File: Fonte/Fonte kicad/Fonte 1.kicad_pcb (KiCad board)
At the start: 2 copper layers, 12 parts, among them J1 Screw_Terminal_01x03, Q1 BC547

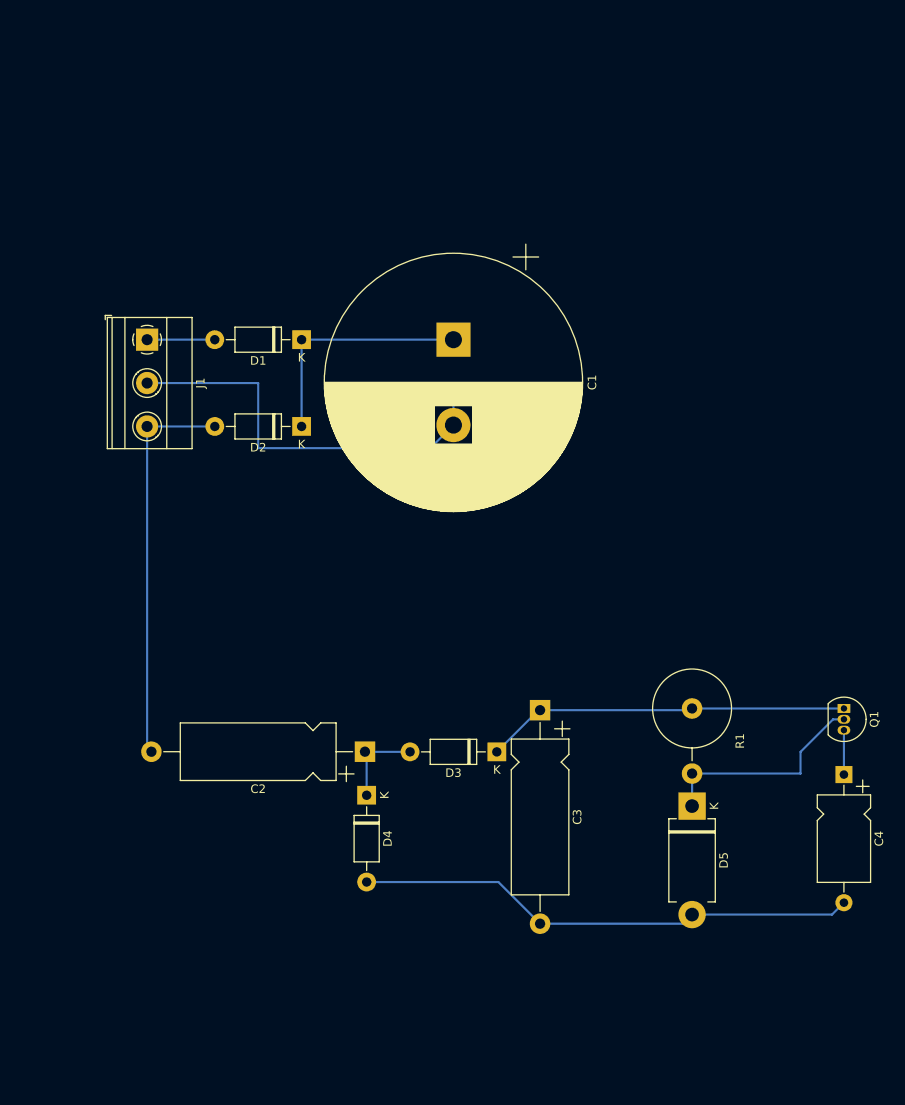
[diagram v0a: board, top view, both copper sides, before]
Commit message: Add files via upload
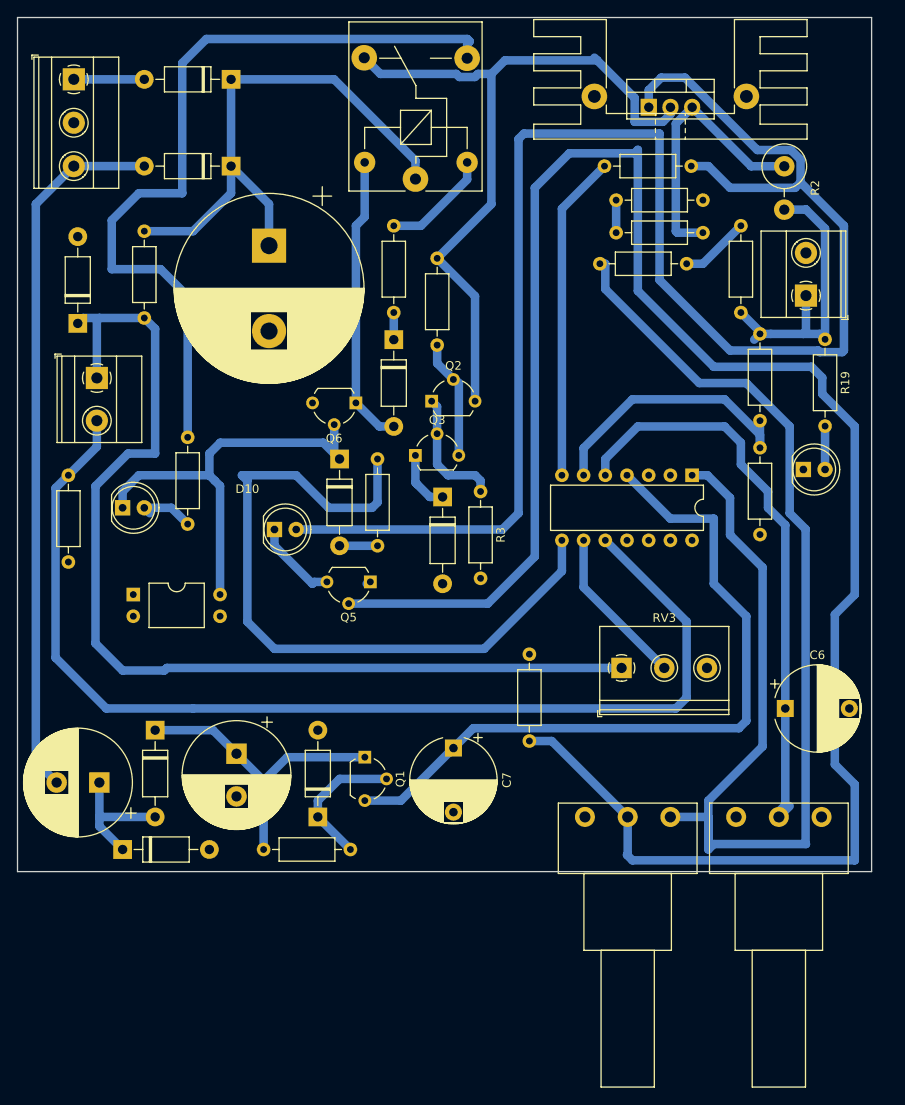
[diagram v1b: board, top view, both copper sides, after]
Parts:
- removed C4: 100n, Capacitor_THT:CP_Axial_L10.0mm_D6.0mm_P15.00mm_Horizontal
- added C6: 10u, Capacitor_THT:CP_Radial_D10.0mm_P7.50mm, F.Cu at (104.9, 88.9)
- added C7: 100n, Capacitor_THT:CP_Radial_D10.0mm_P7.50mm, F.Cu at (66.0, 93.5)
- added D10: LED, LED_THT:LED_D5.0mm, F.Cu at (45.1, 67.9)
- added D11: LED, LED_THT:LED_D5.0mm, F.Cu at (27.3, 65.4)
- added D12: LED, LED_THT:LED_D5.0mm, F.Cu at (107.0, 60.9)
- added D6: 1N53xxB, Diode_THT:D_DO-41_SOD81_P10.16mm_Horizontal, F.Cu at (64.8, 64.1)
- added D7: 1N4007, Diode_THT:D_DO-41_SOD81_P10.16mm_Horizontal, F.Cu at (59.1, 45.7)
- added D8: 1N4007, Diode_THT:D_DO-41_SOD81_P10.16mm_Horizontal, F.Cu at (52.7, 59.7)
- added D9: 1N53xxB, Diode_THT:D_DO-41_SOD81_P10.16mm_Horizontal, F.Cu at (22.1, 43.8)
- added HS1: Heatsink, Heatsink:Heatsink_Stonecold_HS-132_32x14mm_2xFixation1.5mm, F.Cu at (91.4, 17.2)
- added J2: Conn_02x02_Top_Bottom, Package_DIP:DIP-4_W10.16mm, F.Cu at (28.6, 75.6)
- added J3: Screw_Terminal_01x02, TerminalBlock_Phoenix:TerminalBlock_Phoenix_MKDS-1,5-2_1x02_P5.00mm_Horizontal, F.Cu at (107.3, 40.6)
- added J4: Screw_Terminal_01x02, TerminalBlock_Phoenix:TerminalBlock_Phoenix_MKDS-1,5-2_1x02_P5.00mm_Horizontal, F.Cu at (24.3, 50.2)
- added K1: SANYOU_SRD_Form_C, Relay_THT:Relay_SPDT_SANYOU_SRD_Series_Form_C, F.Cu at (61.6, 26.9)
- added Q2: BC556, Package_TO_SOT_THT:TO-92L_Wide, F.Cu at (63.5, 52.9)
- added Q3: BC556, Package_TO_SOT_THT:TO-92L_Wide, F.Cu at (61.6, 59.3)
- added Q4: IRF540N, Package_TO_SOT_THT:TO-220-3_Vertical, F.Cu at (88.9, 18.5)
- added Q5: 2N7000, Package_TO_SOT_THT:TO-92L_Wide, F.Cu at (56.3, 74.1)
- added Q6: BC547, Package_TO_SOT_THT:TO-92L_Wide, F.Cu at (54.6, 53.1)
- added R10: R, Resistor_THT:R_Axial_DIN0207_L6.3mm_D2.5mm_P10.16mm_Horizontal, F.Cu at (74.9, 92.7)
- added R11: R, Resistor_THT:R_Axial_DIN0207_L6.3mm_D2.5mm_P10.16mm_Horizontal, F.Cu at (83.7, 25.4)
- added R12: R, Resistor_THT:R_Axial_DIN0207_L6.3mm_D2.5mm_P10.16mm_Horizontal, F.Cu at (101.9, 45.0)
- added R13: R, Resistor_THT:R_Axial_DIN0207_L6.3mm_D2.5mm_P10.16mm_Horizontal, F.Cu at (21.0, 61.6)
- added R16: R, Resistor_THT:R_Axial_DIN0207_L6.3mm_D2.5mm_P10.16mm_Horizontal, F.Cu at (57.1, 59.7)
- added R17: R, Resistor_THT:R_Axial_DIN0207_L6.3mm_D2.5mm_P10.16mm_Horizontal, F.Cu at (59.1, 42.5)
- added R18: R, Resistor_THT:R_Axial_DIN0207_L6.3mm_D2.5mm_P10.16mm_Horizontal, F.Cu at (29.8, 33.0)
- added R19: R, Resistor_THT:R_Axial_DIN0207_L6.3mm_D2.5mm_P10.16mm_Horizontal, F.Cu at (109.5, 45.7)
- added R2: R_Small, Resistor_THT:R_Axial_DIN0516_L15.5mm_D5.0mm_P5.08mm_Vertical, F.Cu at (104.8, 25.4)
- added R20: R, Resistor_THT:R_Axial_DIN0207_L6.3mm_D2.5mm_P10.16mm_Horizontal, F.Cu at (101.9, 58.4)
- added R3: R, Resistor_THT:R_Axial_DIN0207_L6.3mm_D2.5mm_P10.16mm_Horizontal, F.Cu at (69.2, 63.5)
- added R4: R, Resistor_THT:R_Axial_DIN0207_L6.3mm_D2.5mm_P10.16mm_Horizontal, F.Cu at (34.9, 57.1)
- added R5: R, Resistor_THT:R_Axial_DIN0207_L6.3mm_D2.5mm_P10.16mm_Horizontal, F.Cu at (64.1, 36.2)
- added R6: R, Resistor_THT:R_Axial_DIN0207_L6.3mm_D2.5mm_P10.16mm_Horizontal, F.Cu at (95.2, 33.2)
- added R7: R, Resistor_THT:R_Axial_DIN0207_L6.3mm_D2.5mm_P10.16mm_Horizontal, F.Cu at (99.7, 42.5)
- added R8: R, Resistor_THT:R_Axial_DIN0207_L6.3mm_D2.5mm_P10.16mm_Horizontal, F.Cu at (85.1, 29.4)
- added R9: R, Resistor_THT:R_Axial_DIN0207_L6.3mm_D2.5mm_P10.16mm_Horizontal, F.Cu at (93.3, 36.8)
- added RV1: R_Potentiometer, Potentiometer_THT:Potentiometer_Piher_PC-16_Single_Horizontal, F.Cu at (99.1, 101.6)
- added RV2: R_Potentiometer, Potentiometer_THT:Potentiometer_Piher_PC-16_Single_Horizontal, F.Cu at (81.4, 101.6)
- added RV3: R_Potentiometer, TerminalBlock_Philmore:TerminalBlock_Philmore_TB133_1x03_P5.00mm_Horizontal, F.Cu at (85.7, 84.2)
- added U1: LM324, Package_DIP:DIP-14_W7.62mm, F.Cu at (94.0, 61.6)
- C1: footprint Capacitor_THT:CP_Radial_D30.0mm_P10.00mm_SnapIn -> Capacitor_THT:CP_Radial_D22.0mm_P10.00mm_SnapIn
- C2, C3: footprint Capacitor_THT:CP_Axial_L18.0mm_D6.5mm_P25.00mm_Horizontal -> Capacitor_THT:CP_Radial_D12.5mm_P5.00mm
- D5: footprint Diode_THT:D_DO-201AD_P12.70mm_Horizontal -> Diode_THT:D_DO-41_SOD81_P10.16mm_Horizontal
- Q1: footprint Package_TO_SOT_THT:TO-92_Inline -> Package_TO_SOT_THT:TO-92L_Wide
- R1: footprint Resistor_THT:R_Axial_DIN0918_L18.0mm_D9.0mm_P7.62mm_Vertical -> Resistor_THT:R_Axial_DIN0207_L6.3mm_D2.5mm_P10.16mm_Horizontal
- moved Q1 56.4 mm to (55.7, 94.6)
- moved R1 52.8 mm to (43.8, 105.4), turned to 0 degrees
- moved D5 43.8 mm to (50.2, 101.6), turned to 90 degrees
- moved D3 40.1 mm to (31.1, 91.4), turned to -90 degrees
- moved C3 35.9 mm to (40.6, 94.2)
- moved J1 31.7 mm to (21.6, 15.2)
- moved D2 31.6 mm to (40.0, 25.4)
- moved D1 31.6 mm to (40.0, 15.2)
- moved C2 31.3 mm to (24.6, 97.6)
- moved D4 29.3 mm to (27.3, 105.4), turned to 0 degrees
- moved C1 24.2 mm to (44.5, 34.7)
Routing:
- net Net-(Q5-G): track 0.00 -> 230.1 mm
- net Net-(D10-A): track 0.00 -> 192.7 mm
- net Net-(R9-Pad2): track 0.00 -> 151.8 mm
- net Net-(J4-Pin_2): track 0.00 -> 129.0 mm
- net Net-(D9-K): track 0.00 -> 121.6 mm
- net GND: track 108.4 -> 0.52 mm
- net NO: track 0.00 -> 94.3 mm
- net Net-(Q2-E): track 0.00 -> 86.6 mm
- net Net-(R16-Pad1): track 0.00 -> 85.7 mm
- net VCC: track 5.20 -> 86.0 mm
- net V_ref: track 0.00 -> 69.1 mm
- net Net-(D11-K): track 0.00 -> 50.7 mm
- net Net-(R11-Pad1): track 0.00 -> 38.3 mm
- net V_in: track 46.2 -> 83.3 mm
- net V_ret: track 27.9 -> 64.2 mm
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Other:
- board outline added: 100 x 100 mm
